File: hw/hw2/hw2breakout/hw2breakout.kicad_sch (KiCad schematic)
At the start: 8 parts, among them J1 Conn_01x03_Pin, J2 Conn_01x03_Pin, J3 Conn_01x03_Pin, U1 PCT2075DP

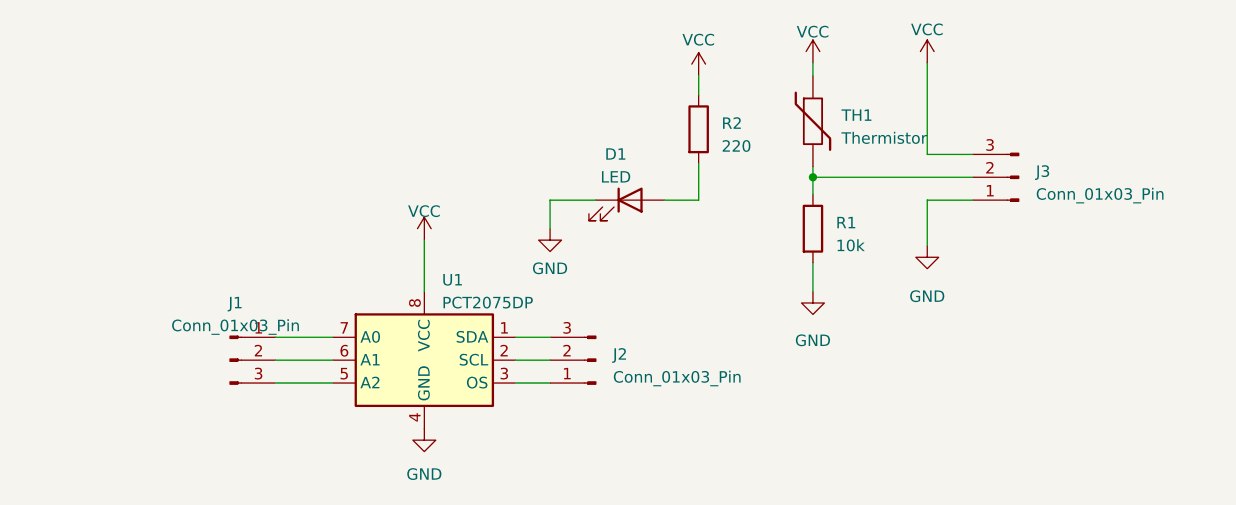
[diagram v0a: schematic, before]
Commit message: rev 2 for hw2
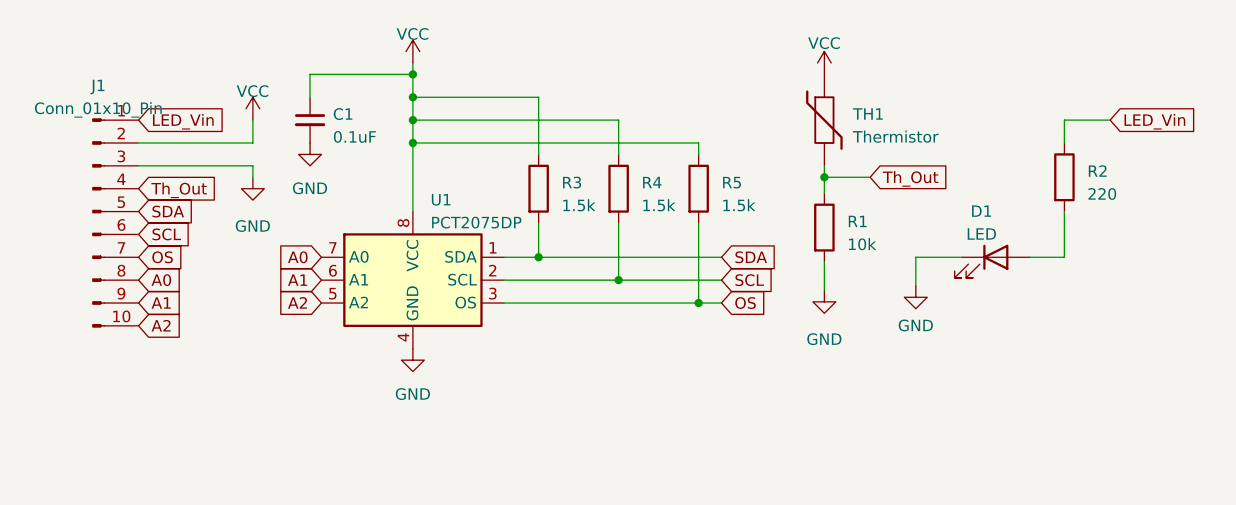
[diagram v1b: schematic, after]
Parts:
- removed J1, J2, J3: Conn_01x03_Pin, Connector_PinHeader_2.54mm:PinHeader_1x03_P2.54mm_Vertical, symbol Connector:Conn_01x03_Pin
- added C1: 0.1uF, Capacitor_THT:C_Disc_D5.0mm_W2.5mm_P2.50mm, symbol Device:C_Small
- added J1: Conn_01x10_Pin, Connector_PinHeader_2.54mm:PinHeader_1x10_P2.54mm_Vertical, symbol Connector:Conn_01x10_Pin
- added R3, R4, R5: 1.5k, Resistor_THT:R_Axial_DIN0207_L6.3mm_D2.5mm_P10.16mm_Horizontal, symbol Device:R
- D1: footprint LED_SMD:LED_0805_2012Metric -> LED_SMD:LED_0805_2012Metric_Pad1.15x1.40mm_HandSolder
- TH1: footprint Resistor_SMD:R_0603_1608Metric -> Resistor_SMD:R_0603_1608Metric_Pad0.98x0.95mm_HandSolder
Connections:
- net GND: now also C1.2, J1.3 (Pin_3)
- net VCC: now also C1.1, J1.2 (Pin_2), R3.1, R4.1, R5.1; no longer R2.1
- net Th_Out: now reaches R1.1, TH1.2
- net Th_Out: now also J1.4 (Pin_4)
- net SDA: now reaches U1.1 (SDA)
- net SDA: now also J1.5 (Pin_5), R3.2
- net SCL: now reaches U1.2 (SCL)
- net SCL: now also J1.6 (Pin_6), R4.2
- net OS: now reaches U1.3 (OS)
- net OS: now also J1.7 (Pin_7), R5.2
- net A2: now reaches U1.5 (A2)
- net A2: now also J1.10 (Pin_10)
- net A1: now reaches U1.6 (A1)
- net A1: now also J1.9 (Pin_9)
- net A0: now reaches U1.7 (A0)
- net A0: now also J1.8 (Pin_8)
- new net LED_Vin: J1.1 (Pin_1), R2.1
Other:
- moved on the sheet: D1, R1, R2, TH1, U1
